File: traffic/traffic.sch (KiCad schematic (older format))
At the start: 8 parts, among them J1 Conn_01x06_Male, J2 Conn_01x02_Male

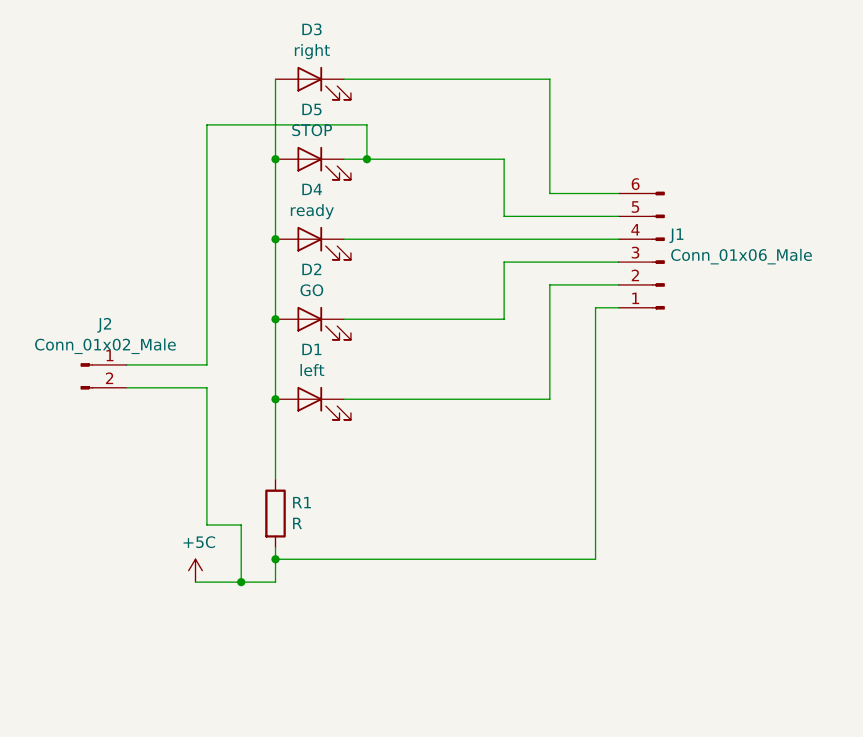
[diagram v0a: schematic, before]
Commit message: gerbers generate
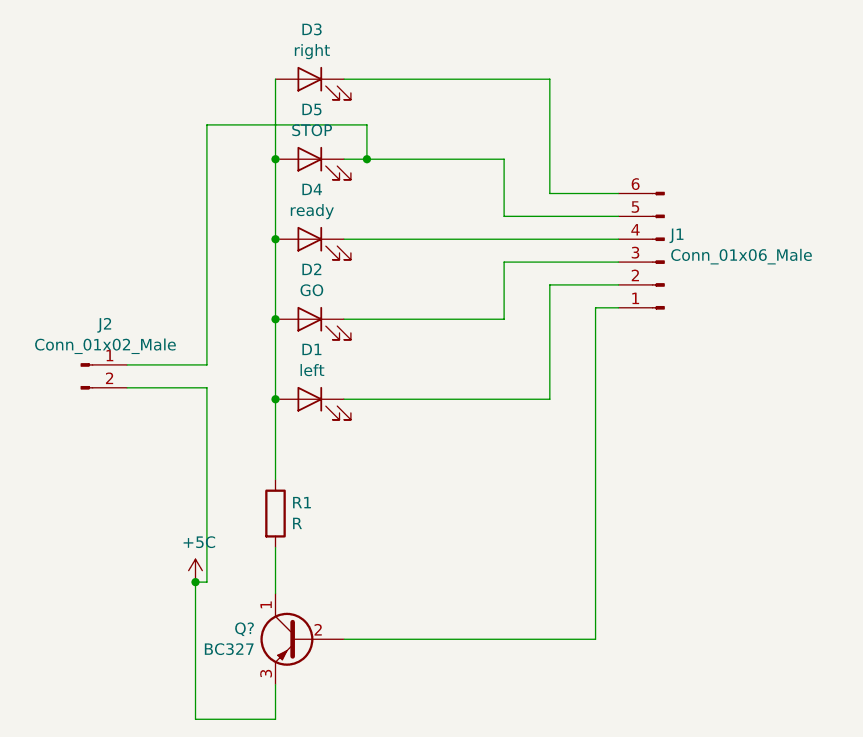
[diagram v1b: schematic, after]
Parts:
- added Q?: BC327, Package_TO_SOT_THT:TO-92_Inline, symbol Transistor_BJT:BC327
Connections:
- net +5C: now also Q?.3 (E); no longer J1.1 (Pin_1), R1.2
- new net: Q?.1 (C), R1.2
- new net: J1.1 (Pin_1), Q?.2 (B)
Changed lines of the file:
@@
 	1    0    0    -1
 $EndComp
-Wire Wire Line
-	5050 4750 5050 4800
 $Comp
 L Connector:Conn_01x06_Male J1
@@
 	-1   0    0    1
 $EndComp
-Wire Wire Line
-	5050 4800 6450 4800
-Wire Wire Line
-	6450 4800 6450 3700
-Connection ~ 5050 4800
-Wire Wire Line
-	5050 4800 5050 4900
 Wire Wire Line
 	6550 3700 6450 3700
@@
 	1    0    0    -1
 $EndComp
-Wire Wire Line
-	4700 4900 4900 4900
 $Comp
 L Connector:Conn_01x02_Male J2
@@
 	4400 4050 4750 4050
 Wire Wire Line
-	4750 4050 4750 4650
-Wire Wire Line
-	4750 4650 4900 4650
-Wire Wire Line
-	4900 4650 4900 4900
-Connection ~ 4900 4900
-Wire Wire Line
-	4900 4900 5050 4900
-Wire Wire Line
 	4400 3950 4750 3950
 Wire Wire Line
@@
 Wire Wire Line
 	5450 3050 6050 3050
+Wire Wire Line
+	6450 3700 6450 5150
+Wire Wire Line
+	6450 5150 5350 5150
+Wire Wire Line
+	5050 4750 5050 4950
+Wire Wire Line
+	4700 4900 4700 5500
+Wire Wire Line
+	4700 5500 5050 5500
+Wire Wire Line
+	5050 5500 5050 5350
+Connection ~ 4700 4900
+Wire Wire Line
+	4700 4900 4750 4900
+Wire Wire Line
+	4750 4050 4750 4900
+$Comp
+L Transistor_BJT:BC327 Q?
+U 1 1 5C480656
+P 5150 5150
+F 0 "Q?" H 5340 5196 50  0000 L CNN
+F 1 "BC327" H 5340 5105 50  0000 L CNN
+F 2 "Package_TO_SOT_THT:TO-92_Inline" H 5350 5075 50  0001 L CIN
+F 3 "http://www.onsemi.com/pub_link/Collateral/BC327-D.PDF" H 5150 5150 50  0001 L CNN
+	1    5150 5150
+	-1   0    0    -1
+$EndComp
 $EndSCHEMATC
